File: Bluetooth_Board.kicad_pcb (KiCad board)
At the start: 4 copper layers, 100 x 50 mm, 71 parts, among them IC2 STM32WB55CGU6, J1 I/O_HDR, J11 BOOT0_Jumper, J2 I2S_OR_LJ_OUT, J24 SWDB, J3 SMA PCB END LAUNCH JACK ROUND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, J4 I2C1_Headers, J5 UART1_HDR, J7 USB_C_Receptacle_USB2.0_16P, Q1 MOSFET_SI2333DDS-T1-BE3, U4 SN74LVC1G07DBVR, U5 USBLC6-2SC6

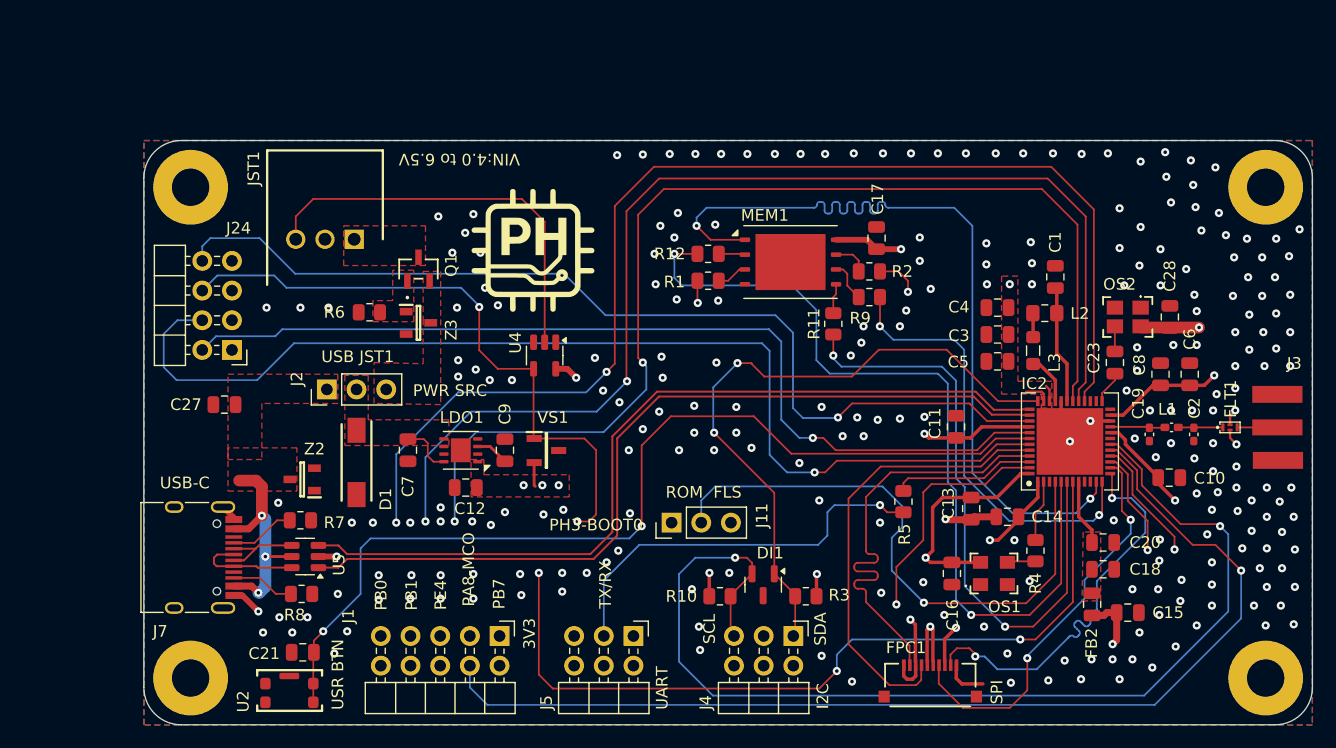
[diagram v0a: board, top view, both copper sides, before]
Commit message: Update
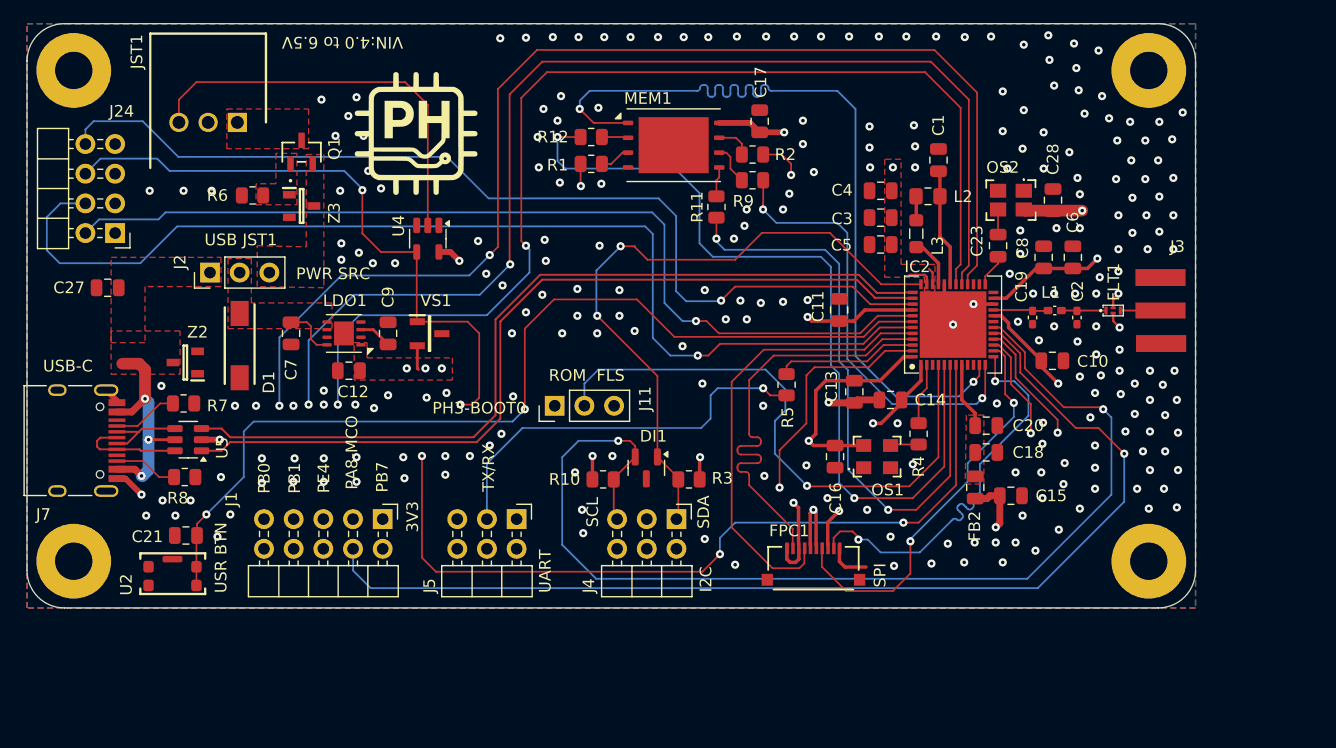
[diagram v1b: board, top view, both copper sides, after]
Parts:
- moved C12 14.1 mm to (127.5, 99.7)
- moved R6 14.1 mm to (119.3, 84.7)
- moved C1 14.1 mm to (178.0, 81.7)
- moved C10 14.1 mm to (187.8, 98.8)
- moved C11 14.1 mm to (169.5, 94.5)
- moved C13 14.1 mm to (170.8, 101.5)
- moved C14 14.1 mm to (173.9, 102.2)
- moved C15 14.1 mm to (184.2, 110.4)
- moved C16 14.1 mm to (169.2, 107.0)
- moved C17 14.1 mm to (162.7, 78.3)
- moved C18 14.1 mm to (182.1, 106.7)
- moved C19 14.1 mm to (186.1, 95.2)
- moved C2 14.1 mm to (189.8, 95.2)
- moved C20 14.1 mm to (182.1, 104.4)
- moved C21 14.1 mm to (113.6, 113.8)
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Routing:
- net GND: track 41.6 -> 215.1 mm
- net +3.3V: track 267.9 -> 128.9 mm
- net /STM32WB55CGU6/BOOT0: track 50.3 -> 157.7 mm
- net /STM32WB55CGU6/PA7_QUADSPI_BK1_IO2: track 71.8 -> 12.5 mm
- net /STM32WB55CGU6/PA6_QUADSPI_BK1_IO3: track 50.3 -> 12.8 mm
- net /Interfaces/I/O_HDR3: track 110.7 -> 97.9 mm
- net /Interfaces/I/O_HDR2: track 107.6 -> 94.8 mm
- net /Interfaces/I/O_HDR4: track 114.7 -> 101.9 mm
- net /Interfaces/NRST: track 129.3 -> 122.5 mm

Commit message: Update
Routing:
- net GND: track 215.1 -> 41.6 mm
- net +3.3V: track 128.9 -> 267.9 mm
- net /STM32WB55CGU6/BOOT0: track 157.7 -> 50.3 mm
- net /STM32WB55CGU6/PA7_QUADSPI_BK1_IO2: track 12.5 -> 71.8 mm
- net /STM32WB55CGU6/PA6_QUADSPI_BK1_IO3: track 12.8 -> 50.3 mm
- net /Interfaces/I/O_HDR3: track 97.9 -> 110.7 mm
- net /Interfaces/I/O_HDR2: track 94.8 -> 107.6 mm
- net /Interfaces/I/O_HDR4: track 101.9 -> 114.7 mm
- net /Interfaces/NRST: track 122.5 -> 129.3 mm
